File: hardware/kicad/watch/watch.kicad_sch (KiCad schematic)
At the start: 23 parts, among them IC13 AP510BFA-CBR, IC2 ICE40UP5K-UWG30ITR, IC8 AKD1500PFC040BA, J1 CX90MWD2G-24P, U15 ET020AM03-HT

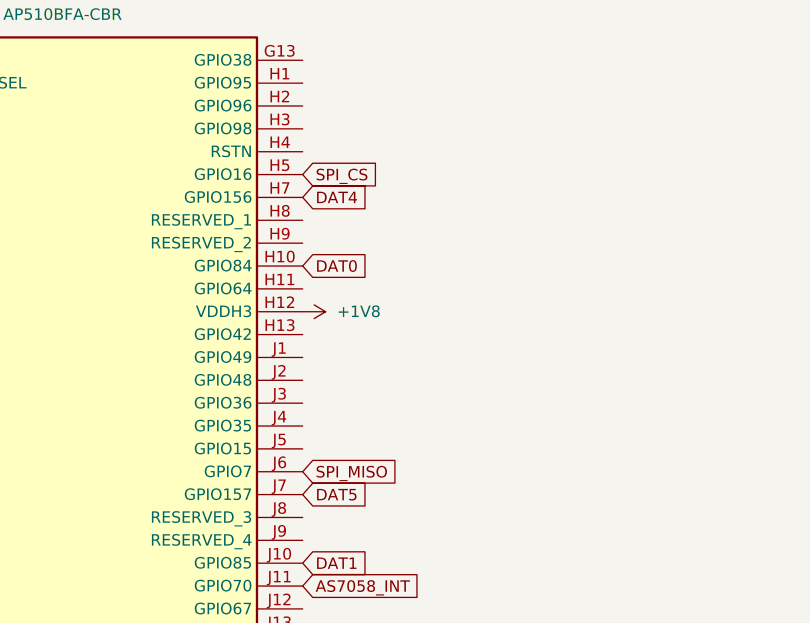
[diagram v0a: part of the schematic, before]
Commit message: fah
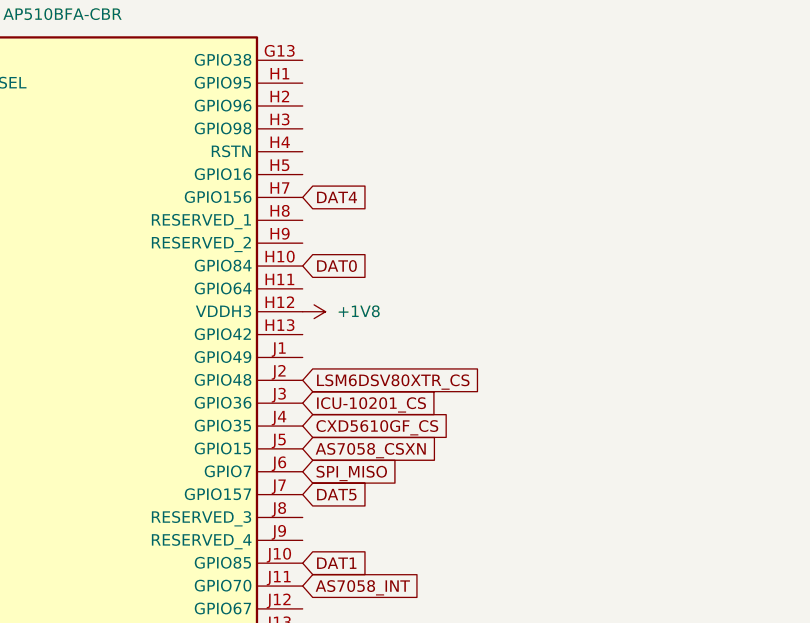
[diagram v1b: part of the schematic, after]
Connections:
- net LSM6DSV80XTR_CS: now reaches IC13.J2 (GPIO48)
- net ICU-10201_CS: now reaches IC13.J3 (GPIO36)
- net CXD5610GF_CS: now reaches IC13.J4 (GPIO35)
- net AS7058_CSXN: now reaches IC13.J5 (GPIO15)
- net SPI_CS: no longer names the net of IC13.H5 (GPIO16)
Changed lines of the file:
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@@
+		)
+	)
+	(global_label "AS7058_CSXN"
+		(shape input)
+		(at 260.35 121.92 0)
+		(fields_autoplaced yes)
+		(effects
+			(font
+				(size 1.27 1.27)
+			)
+			(justify left)
+		)
+		(property "Intersheetrefs" "${INTERSHEET_REFS}"
+			(at 276.4584 121.92 0)
+			(show_name no)
+			(do_not_autoplace no)
+			(effects
+				(font
+					(size 1.27 1.27)
+				)
+				(justify left)
+			)
+		)
+	)
+	(global_label "CXD5610GF_CS"
+		(shape input)
+		(at 260.35 119.38 0)
+		(fields_autoplaced yes)
+		(effects
+			(font
+				(size 1.27 1.27)
+			)
+			(justify left)
+		)
+		(property "Intersheetrefs" "${INTERSHEET_REFS}"
+			(at 277.7284 119.38 0)
+			(show_name no)
+			(do_not_autoplace no)
+			(effects
+				(font
+					(size 1.27 1.27)
+				)
+				(justify left)
+			)
+		)
+	)
+	(global_label "ICU-10201_CS"
+		(shape input)
+		(at 260.35 116.84 0)
+		(fields_autoplaced yes)
+		(effects
+			(font
+				(size 1.27 1.27)
+			)
+			(justify left)
+		)
+		(property "Intersheetrefs" "${INTERSHEET_REFS}"
+			(at 277.6075 116.84 0)
+			(show_name no)
+			(do_not_autoplace no)
+			(effects
+				(font
+					(size 1.27 1.27)
+				)
+				(justify left)
+			)
 		)
 	)
@@
 		)
 	)
+	(global_label "LSM6DSV80XTR_CS"
+		(shape input)
+		(at 260.35 114.3 0)
+		(fields_autoplaced yes)
+		(effects
+			(font
+				(size 1.27 1.27)
+			)
+			(justify left)
+		)
+		(property "Intersheetrefs" "${INTERSHEET_REFS}"
+			(at 281.115 114.3 0)
+			(show_name no)
+			(do_not_autoplace no)
+			(effects
+				(font
+					(size 1.27 1.27)
+				)
+				(justify left)
+			)
+		)
+	)
 	(global_label "AS7058_INT"
 		(shape input)
@@
 			(show_name no)
 			(do_not_autoplace no)
-			(effects
-				(font
-					(size 1.27 1.27)
-				)
-				(justify left)
-			)
-		)
-	)
-	(global_label "SPI_CS"
-		(shape input)
-		(at 260.35 91.44 0)
-		(fields_autoplaced yes)
-		(effects
-			(font
-				(size 1.27 1.27)
-			)
-			(justify left)
-		)
-		(property "Intersheetrefs" "${INTERSHEET_REFS}"
-			(at 269.8666 91.44 0)
-			(show_name no)
-			(do_not_autoplace no)
